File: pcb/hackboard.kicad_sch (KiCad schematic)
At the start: 254 parts, among them SW1 SW_Push_45deg, SW10 SW_Push_45deg, SW11 SW_Push_45deg, SW12 SW_Push_45deg, SW13 SW_Push_45deg, SW14 SW_Push_45deg, SW15 SW_Push_45deg, SW16 SW_Push_45deg, SW17 SW_Push_45deg, SW18 SW_Push_45deg, SW19 SW_Push_45deg, SW2 SW_Push_45deg, SW20 SW_Push_45deg, SW21 SW_Push_45deg, SW22 SW_Push_45deg, SW23 SW_Push_45deg, SW24 SW_Push_45deg, SW25 SW_Push_45deg, SW26 SW_Push_45deg, SW27 SW_Push_45deg, SW28 SW_Push_45deg, SW29 SW_Push_45deg, SW3 SW_Push_45deg, SW30 SW_Push_45deg, SW31 SW_Push_45deg, SW32 SW_Push_45deg, SW33 SW_Push_45deg, SW34 SW_Push_45deg, SW35 SW_Push_45deg, SW36 SW_Push_45deg, SW37 SW_Push_45deg, SW38 SW_Push_45deg, SW39 SW_Push_45deg, SW4 SW_Push_45deg, SW40 SW_Push_45deg, SW41 SW_Push_45deg, SW42 SW_Push_45deg, SW43 SW_Push_45deg, SW44 SW_Push_45deg, SW45 SW_Push_45deg, SW46 SW_Push_45deg, SW47 SW_Push_45deg, SW48 SW_Push_45deg, SW49 SW_Push_45deg, SW5 SW_Push_45deg, SW50 SW_Push_45deg, SW51 SW_Push_45deg, SW52 SW_Push_45deg, SW53 SW_Push_45deg, SW54 SW_Push_45deg, SW55 SW_Push_45deg, SW56 SW_Push_45deg, SW57 SW_Push_45deg, SW58 SW_Push_45deg, SW59 SW_Push_45deg, SW6 SW_Push_45deg, SW60 SW_Push_45deg, SW61 SW_Push_45deg, SW62 SW_Push_45deg, SW63 SW_Push_45deg, SW64 SW_Push_45deg, SW65 SW_Push_45deg, SW66 SW_Push_45deg, SW67 SW_Push_45deg, SW68 SW_Push_45deg, SW69 SW_Push_45deg, SW7 SW_Push_45deg, SW70 SW_Push_45deg, SW71 SW_Push_45deg, SW72 SW_Push_45deg, SW73 SW_Push_45deg, SW74 SW_Push_45deg, SW75 SW_Push_45deg, SW76 SW_Push_45deg, SW77 SW_Push_45deg, SW78 SW_Push_45deg, SW79 SW_Push_45deg, SW8 SW_Push_45deg, SW80 SW_Push_45deg, SW81 SW_Push_45deg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

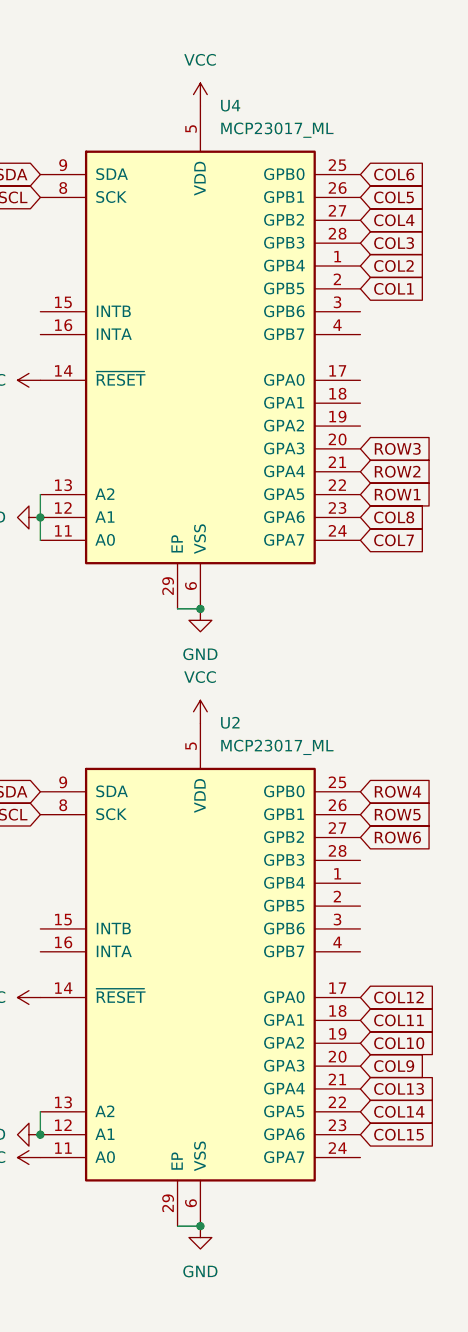
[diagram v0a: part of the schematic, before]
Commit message: modified:   pcb/hackboard.kicad_pcb 	modified:   pcb/hackboard.kicad_prl 	modified:   pcb/hackboard.kicad_sch 	modified:   pcb/production/bom.csv 	modified:   pcb/production/hackboard.zip 	modified:   pcb/production/netlist.ipc 	modified:   pcb/production/positions.csv
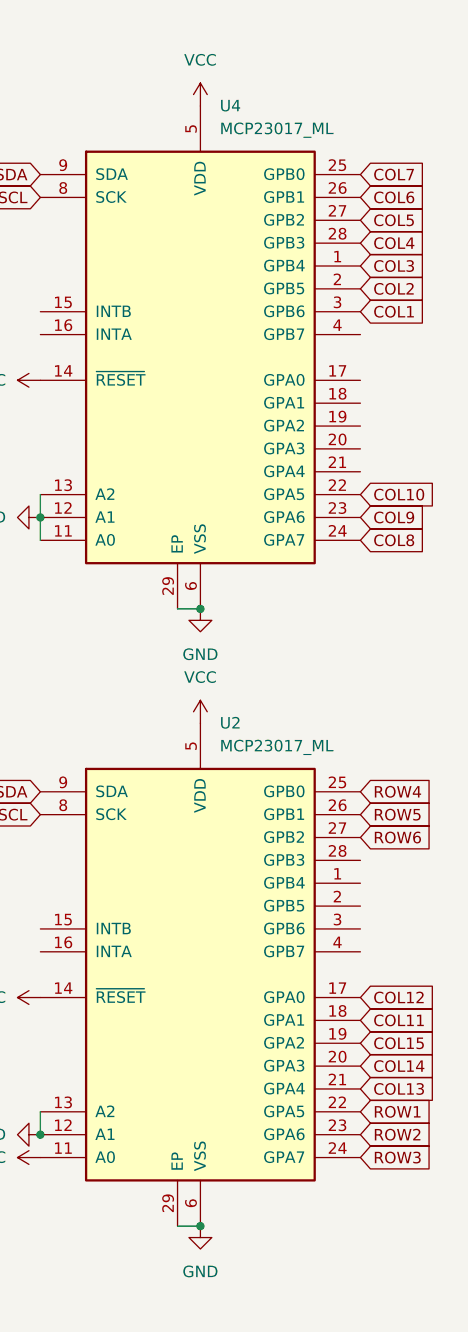
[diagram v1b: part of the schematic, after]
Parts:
- D1, D10, D11, D12, D13, D14, D15, D16, D17, D18, D19, D2, D20, D21, D22, D23, D24, D25, D26, D27, D28, D29, D3, D30, D31, D32, D33, D34, D35, D36, D37, D38, D39, D4, D40, D41, D42, D43, D44, D45, D46, D47, D48, D49, D5, D50, D51, D52, D53, D54, D55, D56, D57, D58, D59, D6, D60, D61, D62, D63, D64, D65, D66, D67, D68, D69, D7, D70, D71, D72, D73, D74, D75, D76, D77, D78, D79, D8, D80, D81, D82, D9: footprint customDiode:D_0402_1005Metric_Pad0.77x0.64mm_HandSolder-withVia -> Diode_SMD:D_SOD-123
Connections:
- net COL1: now also U4.3 (GPB6); no longer U4.2 (GPB5)
- net COL10: now also U4.22 (GPA5); no longer U2.19 (GPA2)
- net COL14: now also U2.20 (GPA3); no longer U2.22 (GPA5)
- net COL15: now also U2.19 (GPA2); no longer U2.23 (GPA6)
- net COL2: now also U4.2 (GPB5); no longer U4.1 (GPB4)
- net COL3: now also U4.1 (GPB4); no longer U4.28 (GPB3)
- net COL4: now also U4.28 (GPB3); no longer U4.27 (GPB2)
- net COL5: now also U4.27 (GPB2); no longer U4.26 (GPB1)
- net COL6: now also U4.26 (GPB1); no longer U4.25 (GPB0)
- net COL7: now also U4.25 (GPB0); no longer U4.24 (GPA7)
- net COL8: now also U4.24 (GPA7); no longer U4.23 (GPA6)
- net COL9: now also U4.23 (GPA6); no longer U2.20 (GPA3)
- net ROW1: now also U2.22 (GPA5); no longer U4.22 (GPA5)
- net ROW2: now also U2.23 (GPA6); no longer U4.21 (GPA4)
- net ROW3: now also U2.24 (GPA7); no longer U4.20 (GPA3)
